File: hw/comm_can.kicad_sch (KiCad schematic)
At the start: 22 parts, among them IC601 ADM3055EBRIZ, J601 43650-0427, J602 43650-0427

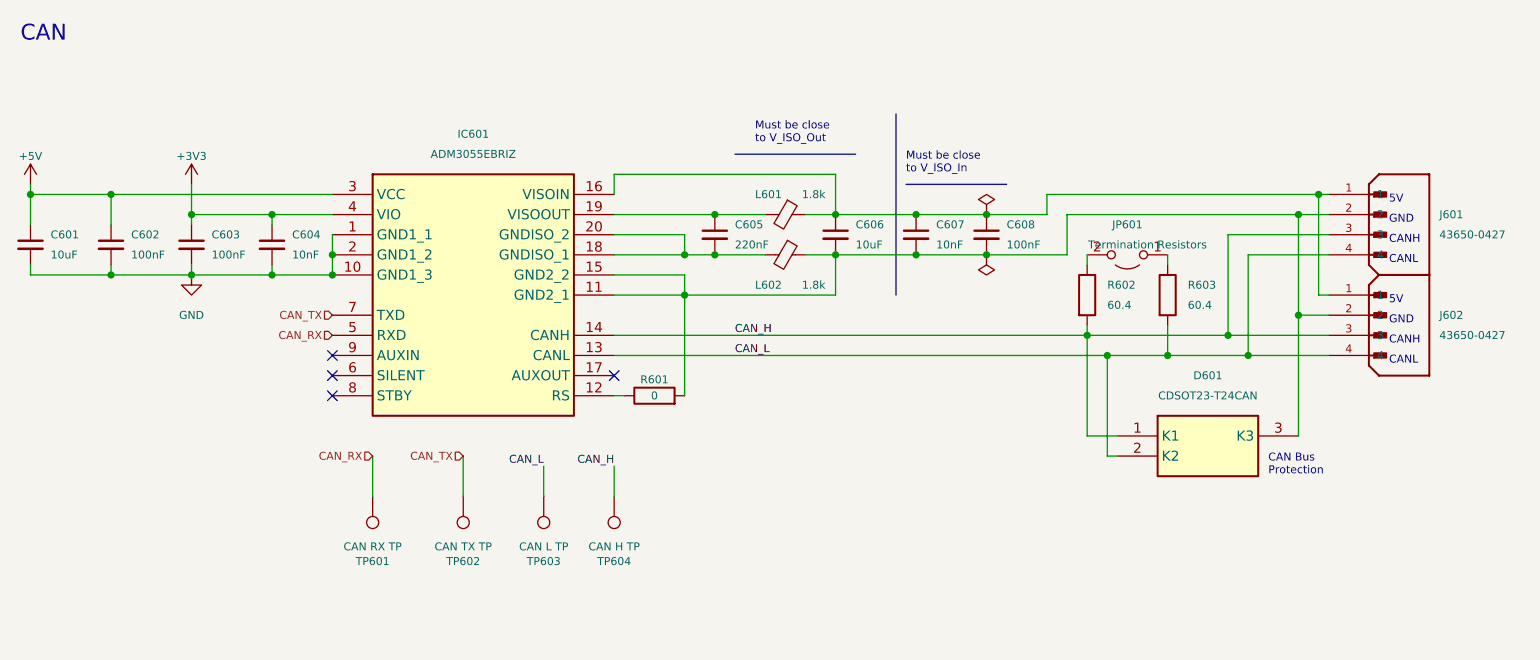
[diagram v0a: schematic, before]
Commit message: init sch changes
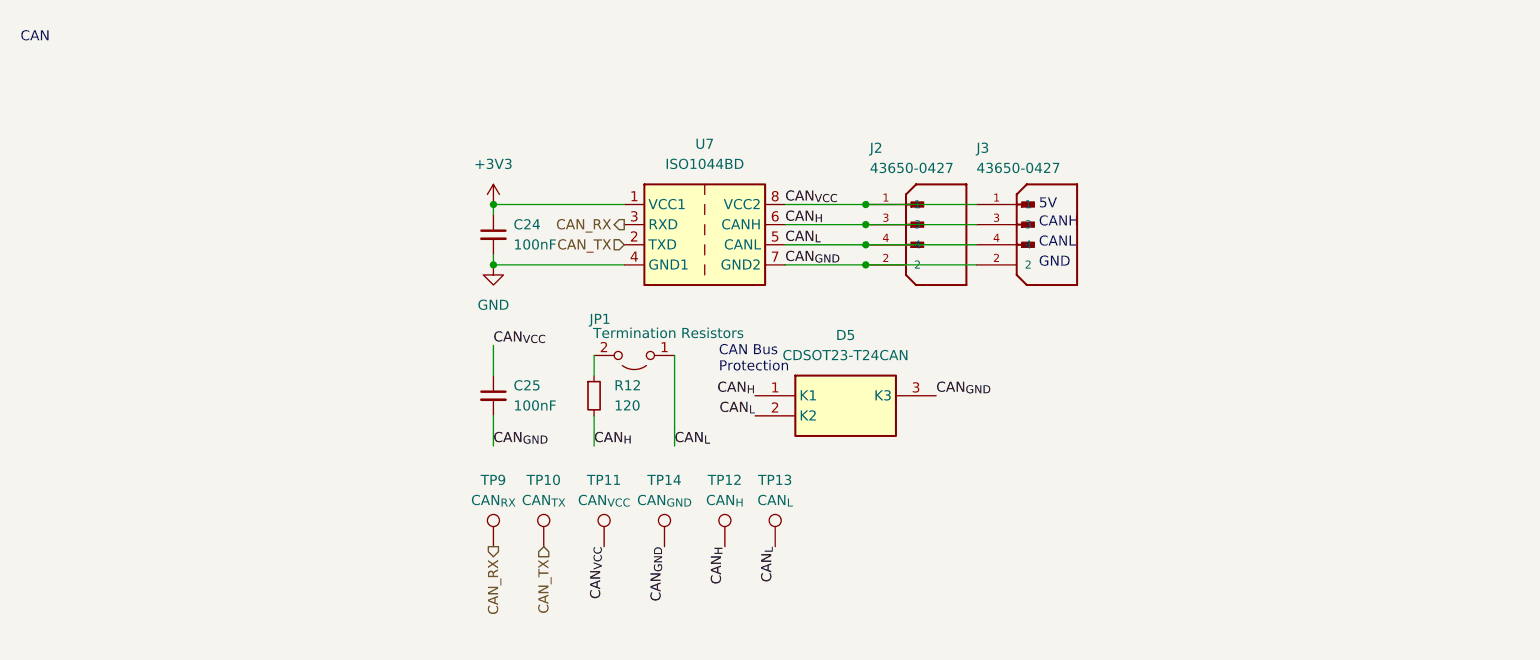
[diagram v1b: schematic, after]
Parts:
- removed C601, C606: 10uF, Capacitor_SMD:C_0402_1005Metric, symbol Device:C_Small
- removed C602, C603, C608: 100nF, Capacitor_SMD:C_0402_1005Metric, symbol Device:C_Small
- removed C604, C607: 10nF, Capacitor_SMD:C_0402_1005Metric, symbol Device:C_Small
- removed C605: 220nF, Capacitor_SMD:C_0402_1005Metric, symbol Device:C_Small
- removed D601: CDSOT23-T24CAN, footprints:bourns_CDSOT23_T24CAN, symbol bourns_CDSOT23_T24CAN:CDSOT23-T24CAN
- removed IC601: ADM3055EBRIZ, footprints:analog_ADM3055EBRIZ, symbol analog_ADM3055EBRIZ:ADM3055EBRIZ
- removed J601, J602: 43650-0427, footprints:molex_microfit_43650_0427, symbol molex_microfit_43650_0427:43650-0427
- removed JP601: Termination Resistors, Connector_PinHeader_2.54mm:PinHeader_1x02_P2.54mm_Vertical, symbol Jumper:Jumper_2_Open
- removed L601, L602: 1.8k, Inductor_SMD:L_0402_1005Metric, symbol Device:FerriteBead_Small
- removed R601: 0, Resistor_SMD:R_0402_1005Metric, symbol Device:R
- removed R602, R603: 60.4, Resistor_SMD:R_0402_1005Metric, symbol Device:R
- removed TP601: CAN RX TP, TestPoint:TestPoint_Pad_1.0x1.0mm, symbol Connector:TestPoint
- removed TP602: CAN TX TP, TestPoint:TestPoint_Pad_1.0x1.0mm, symbol Connector:TestPoint
- removed TP603: CAN L TP, TestPoint:TestPoint_Pad_1.0x1.0mm, symbol Connector:TestPoint
- removed TP604: CAN H TP, TestPoint:TestPoint_Pad_1.0x1.0mm, symbol Connector:TestPoint
- added C24, C25: 100nF, symbol Device:C_Small
- added D5: CDSOT23-T24CAN, footprints:bourns_CDSOT23_T24CAN, symbol bourns_CDSOT23_T24CAN:CDSOT23-T24CAN
- added J2, J3: 43650-0427, footprints:molex_microfit_43650_0427, symbol molex_microfit_43650_0427:43650-0427
- added JP1: Termination Resistors, Connector_PinHeader_2.54mm:PinHeader_1x02_P2.54mm_Vertical, symbol Jumper:Jumper_2_Open
- added R12: 120, symbol Device:R_Small
- added TP10: CAN_{TX}, symbol Connector:TestPoint
- added TP11: CAN_{VCC}, symbol Connector:TestPoint
- added TP12: CAN_{H}, symbol Connector:TestPoint
- added TP13: CAN_{L}, symbol Connector:TestPoint
- added TP14: CAN_{GND}, symbol Connector:TestPoint
- added TP9: CAN_{RX}, symbol Connector:TestPoint
- added U7: ISO1044BD, Package_SO:SOIC-8_3.9x4.9mm_P1.27mm, symbol Interface_CAN_LIN:ISO1044BD
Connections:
- net +3V3: now also C24.1, U7.1 (VCC1)
- net CAN_RX: now also TP9.1, U7.3 (RXD)
- net CAN_TX: now also TP10.1, U7.2 (TXD)
- net GND: now also C24.2, U7.4 (GND1)
- new net: JP1.2 (B), R12.1
- new net CAN_{GND}: C25.2, D5.3 (K3), J2.2, J3.2, TP14.1, U7.7 (GND2)
- new net CAN_{H}: D5.1 (K1), J2.3, J3.3, R12.2, TP12.1, U7.6 (CANH)
- new net CAN_{L}: D5.2 (K2), J2.4, J3.4, JP1.1 (A), TP13.1, U7.5 (CANL)
- new net CAN_{VCC}: C25.1, J2.1, J3.1, TP11.1, U7.8 (VCC2)
- no-connect marks 4 -> 0
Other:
- note removed: "Must be close to V_ISO_In"
- note removed: "Must be close to V_ISO_Out"
